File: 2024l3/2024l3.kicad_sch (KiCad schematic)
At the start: 27 parts, among them J1 Conn_01x06, J2 TOF 0, J3 TOF 1, J4 TOF 2, J5 TOF 3, SW1 SW_SPDT, SW2 SW_SPDT, SW3 SW_SPDT, U1 OpenMV, U2 4754, U3 xiao-esp32c3, U4 Adafruit Featherwing, U7 Teensy 4.0

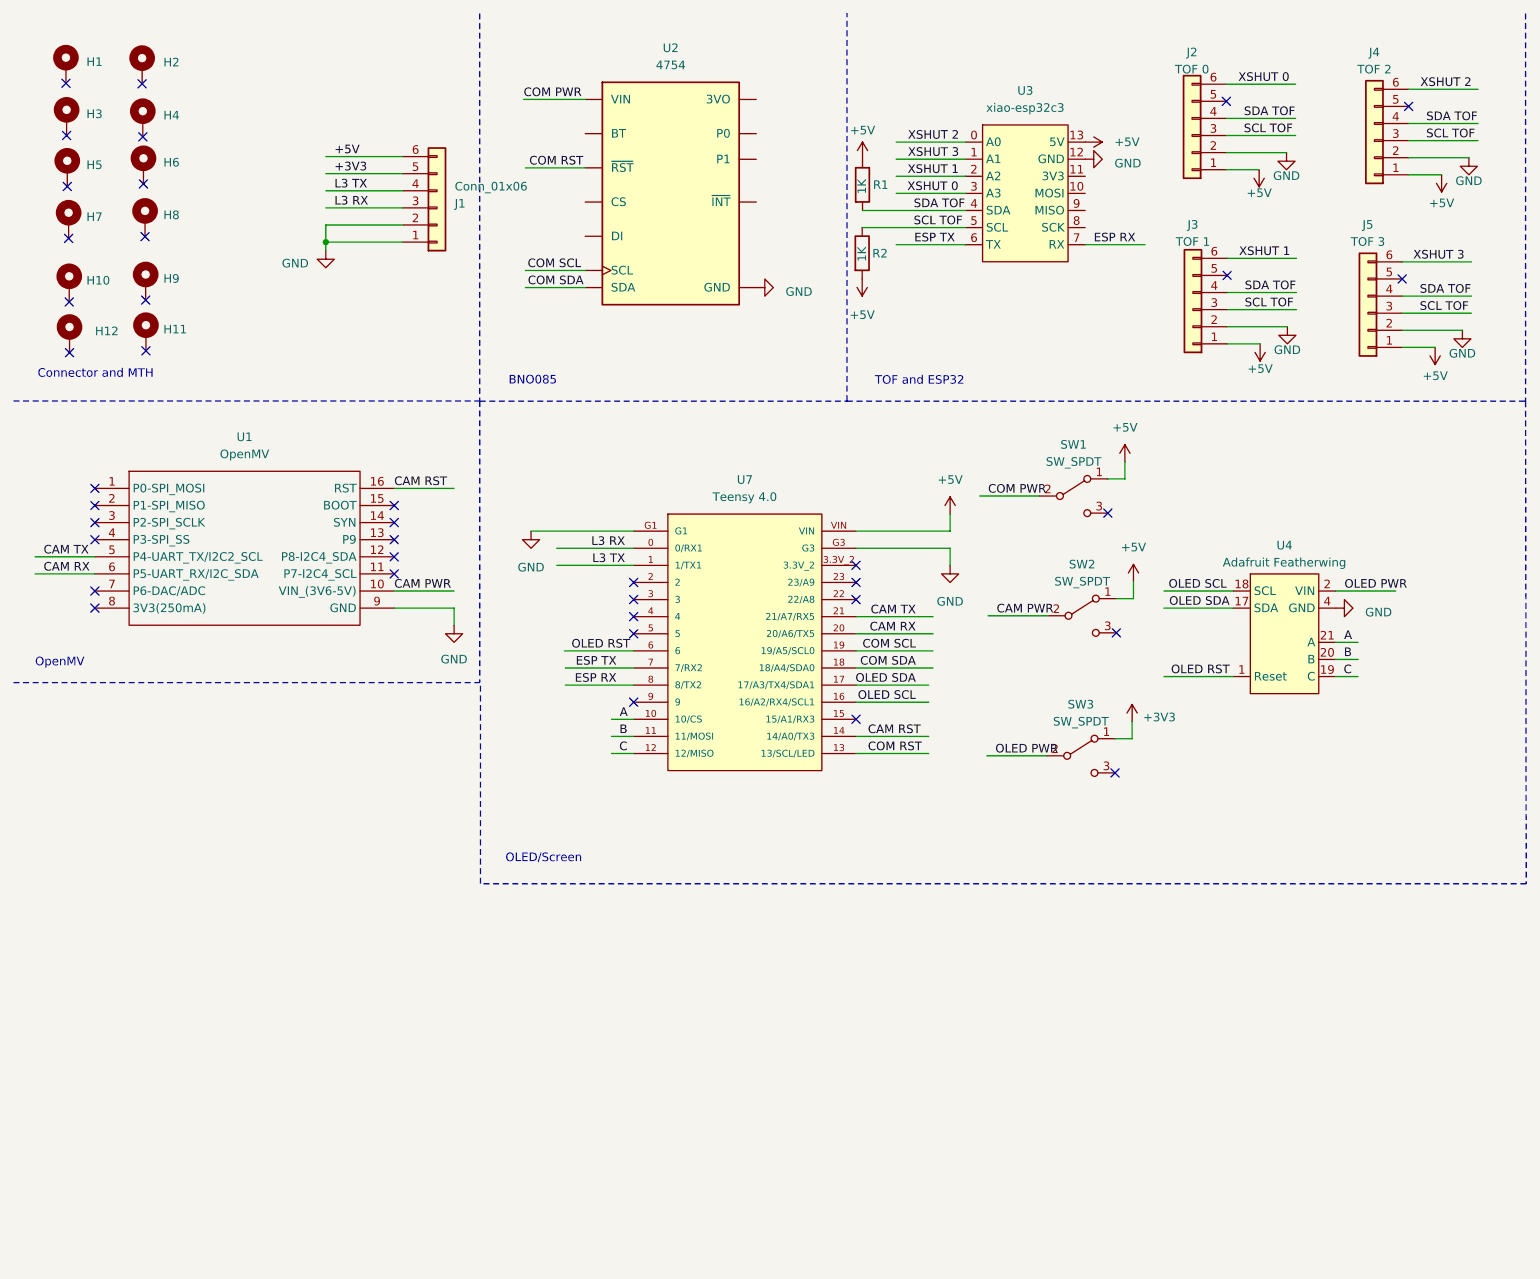
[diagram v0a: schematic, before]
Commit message: L3 Redo
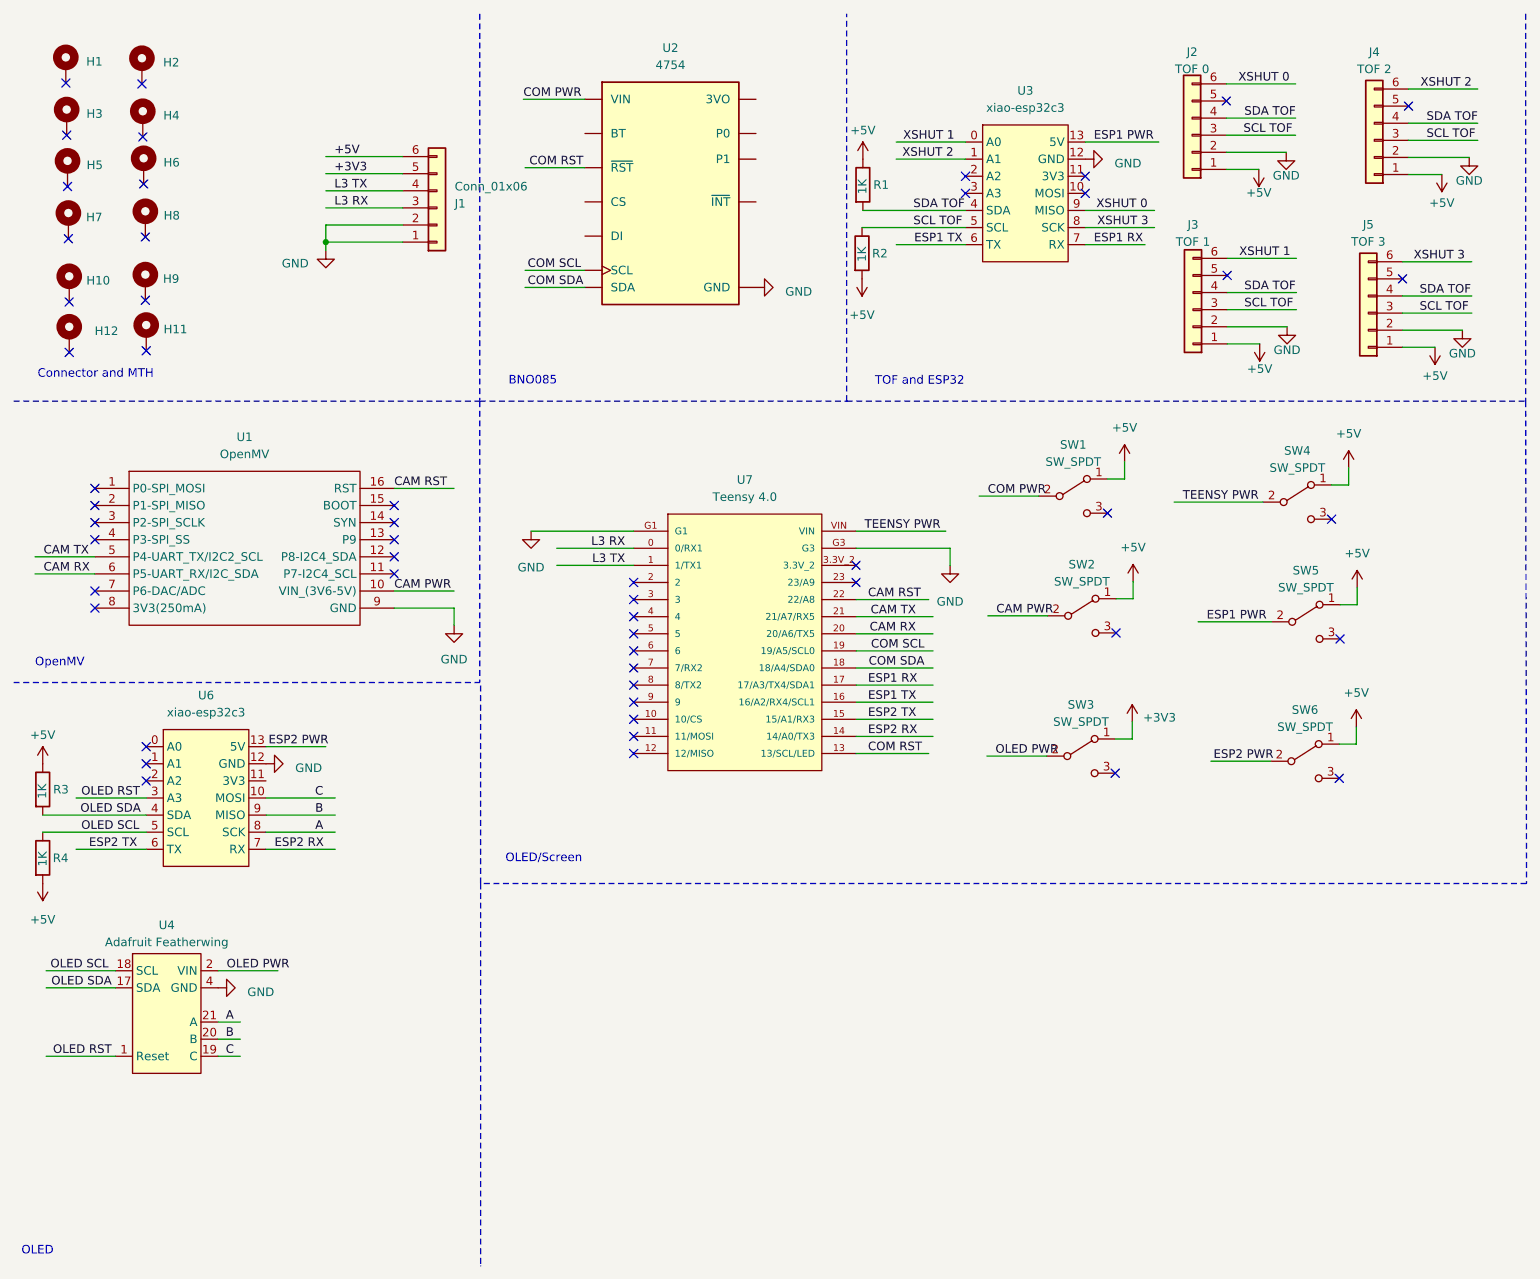
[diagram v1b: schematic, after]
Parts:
- added R3, R4: 1K, 2024l3:res0603, symbol Device:R
- added SW4, SW5, SW6: SW_SPDT, 2024l3:SS12D00G3, symbol Switch:SW_SPDT
- added U6: xiao-esp32c3, 2024l3:xiao-esp32c3, symbol vincent:xiao-esp32c3
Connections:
- net +5V: now also R3.1, R4.2, SW4.1 (A), SW5.1 (A), SW6.1 (A); no longer U3.13 (5V), U7.VIN
- net A: now also U6.8 (SCK); no longer U7.10 (10/CS)
- net B: now also U6.9 (MISO); no longer U7.11 (11/MOSI)
- net C: now also U6.10 (MOSI); no longer U7.12 (12/MISO)
- net CAM RST: now also U7.22 (22/A8); no longer U7.14 (14/A0/TX3)
- net GND: now also U6.12 (GND)
- net OLED RST: now also U6.3 (A3); no longer U7.6
- net OLED SCL: now also R4.1, U6.5 (SCL); no longer U7.16 (16/A2/RX4/SCL1)
- net OLED SDA: now also R3.2, U6.4 (SDA); no longer U7.17 (17/A3/TX4/SDA1)
- net XSHUT 0: now also U3.9 (MISO); no longer U3.3 (A3)
- net XSHUT 1: now also U3.0 (A0); no longer U3.2 (A2)
- net XSHUT 2: now also U3.1 (A1); no longer U3.0 (A0)
- net XSHUT 3: now also U3.8 (SCK); no longer U3.1 (A1)
- net ESP2 TX: now reaches U7.15 (15/A1/RX3)
- net ESP2 TX: now also U6.6 (TX)
- net ESP RX: no longer names the net of U7.8 (8/TX2)
- net ESP RX: no longer U3.7 (RX)
- net ESP TX: no longer names the net of U7.7 (7/RX2)
- net ESP TX: no longer U3.6 (TX)
- new net ESP1 PWR: SW5.2 (B), U3.13 (5V)
- new net ESP1 RX: U3.7 (RX), U7.17 (17/A3/TX4/SDA1)
- new net ESP1 TX: U3.6 (TX), U7.16 (16/A2/RX4/SCL1)
- new net ESP2 PWR: SW6.2 (B), U6.13 (5V)
- new net ESP2 RX: U6.7 (RX), U7.14 (14/A0/TX3)
- new net TEENSY PWR: SW4.2 (B), U7.VIN
- no-connect marks 39 -> 53
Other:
- note added: "OLED"
- moved on the sheet: U4

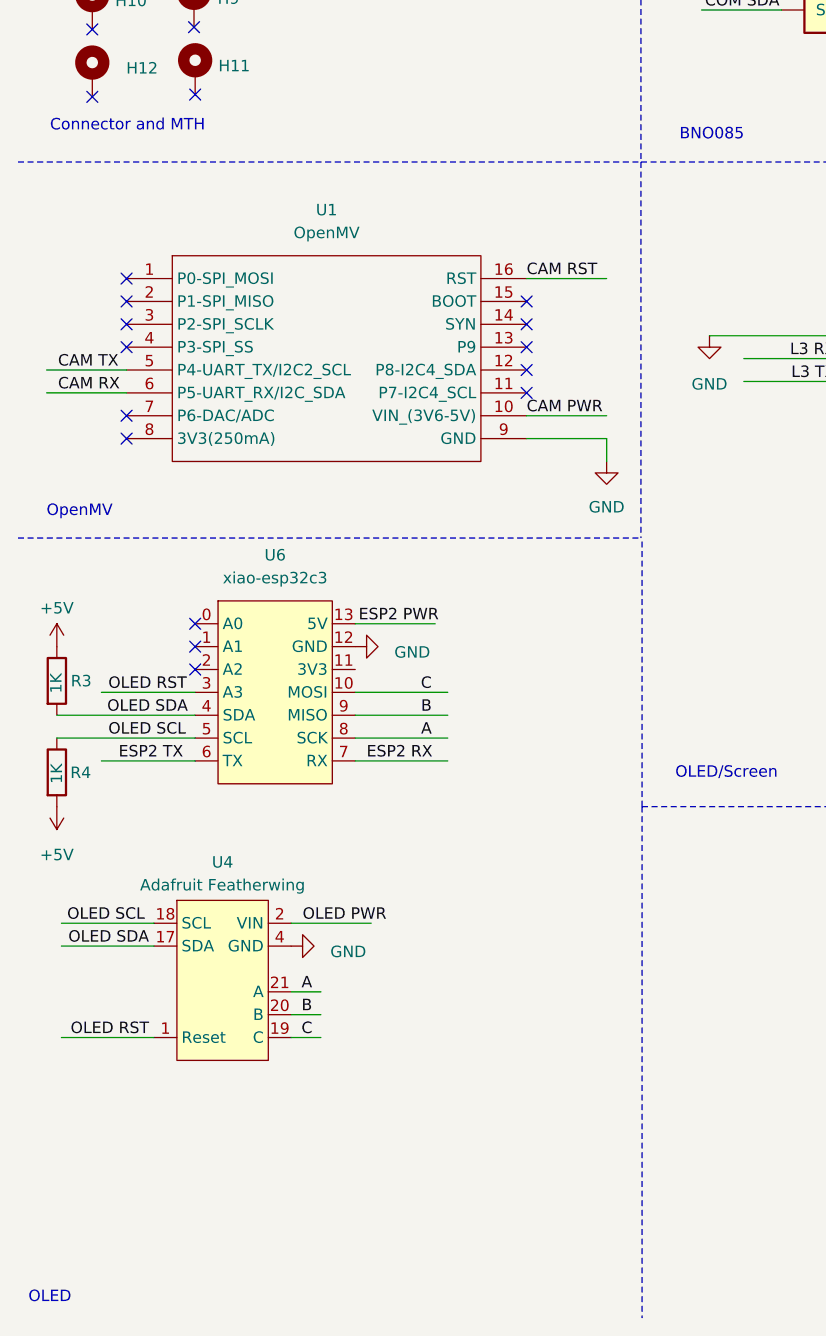
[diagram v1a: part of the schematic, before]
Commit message: Changed OPENMV FOOTPRINT
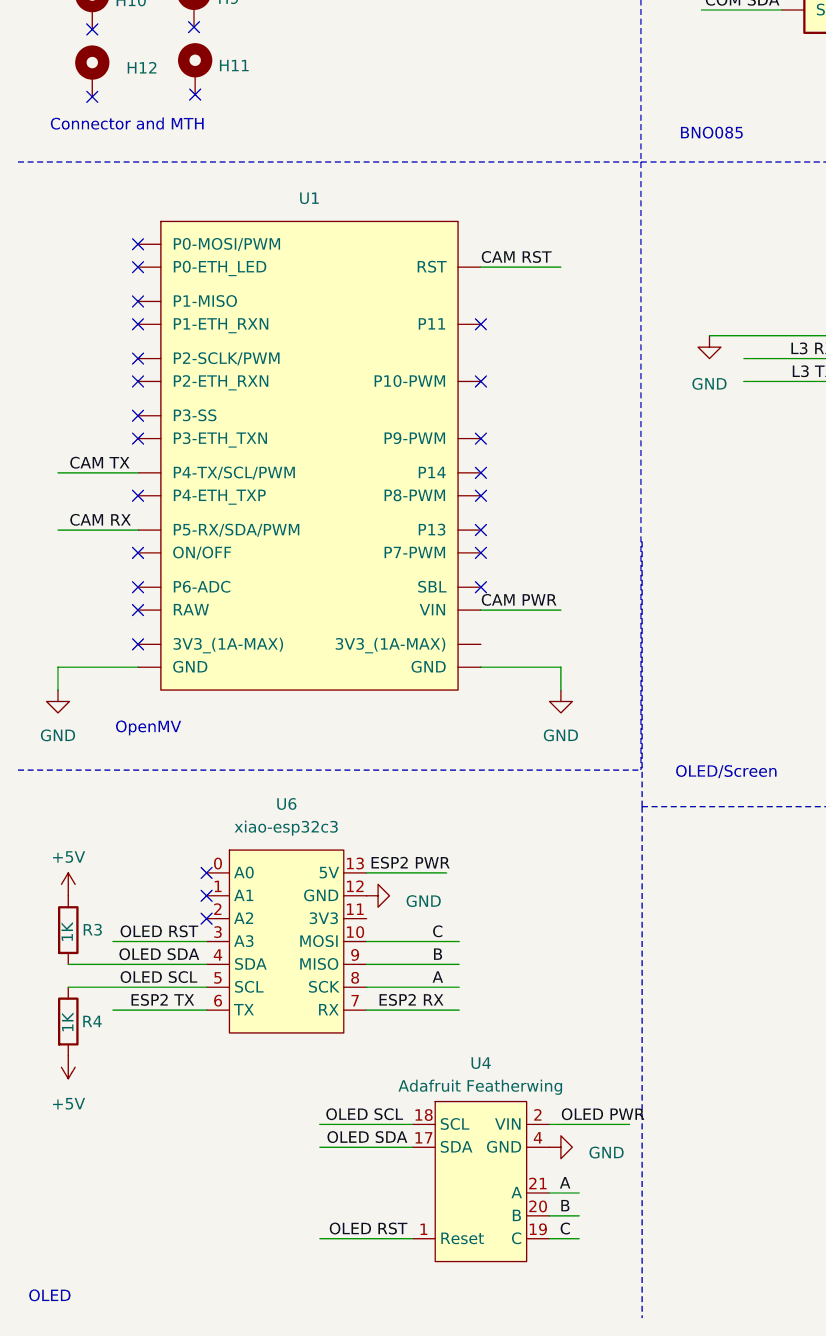
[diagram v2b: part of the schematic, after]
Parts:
- removed U1: OpenMV, 2024l3:openmv, symbol vincent:OpenMV
- added U1: ~, 2024l3:OpenMV_RT, symbol vincent:OpenMV_RT
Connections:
- net CAM PWR: now also U1.29 (VIN)
- net CAM RST: now also U1.17 (RST)
- net CAM RX: now also U1.10 (P5-RX/SDA/PWM)
- net CAM TX: now also U1.8 (P4-TX/SCL/PWM)
- net GND: now also U1.15 (GND), U1.31 (GND)
- no-connect marks 53 -> 63
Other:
- moved on the sheet: R3, R4, U4, U6
